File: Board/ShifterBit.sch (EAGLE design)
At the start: 13 parts, among them P1 PINHD-1X10, P2 PINHD-1X10

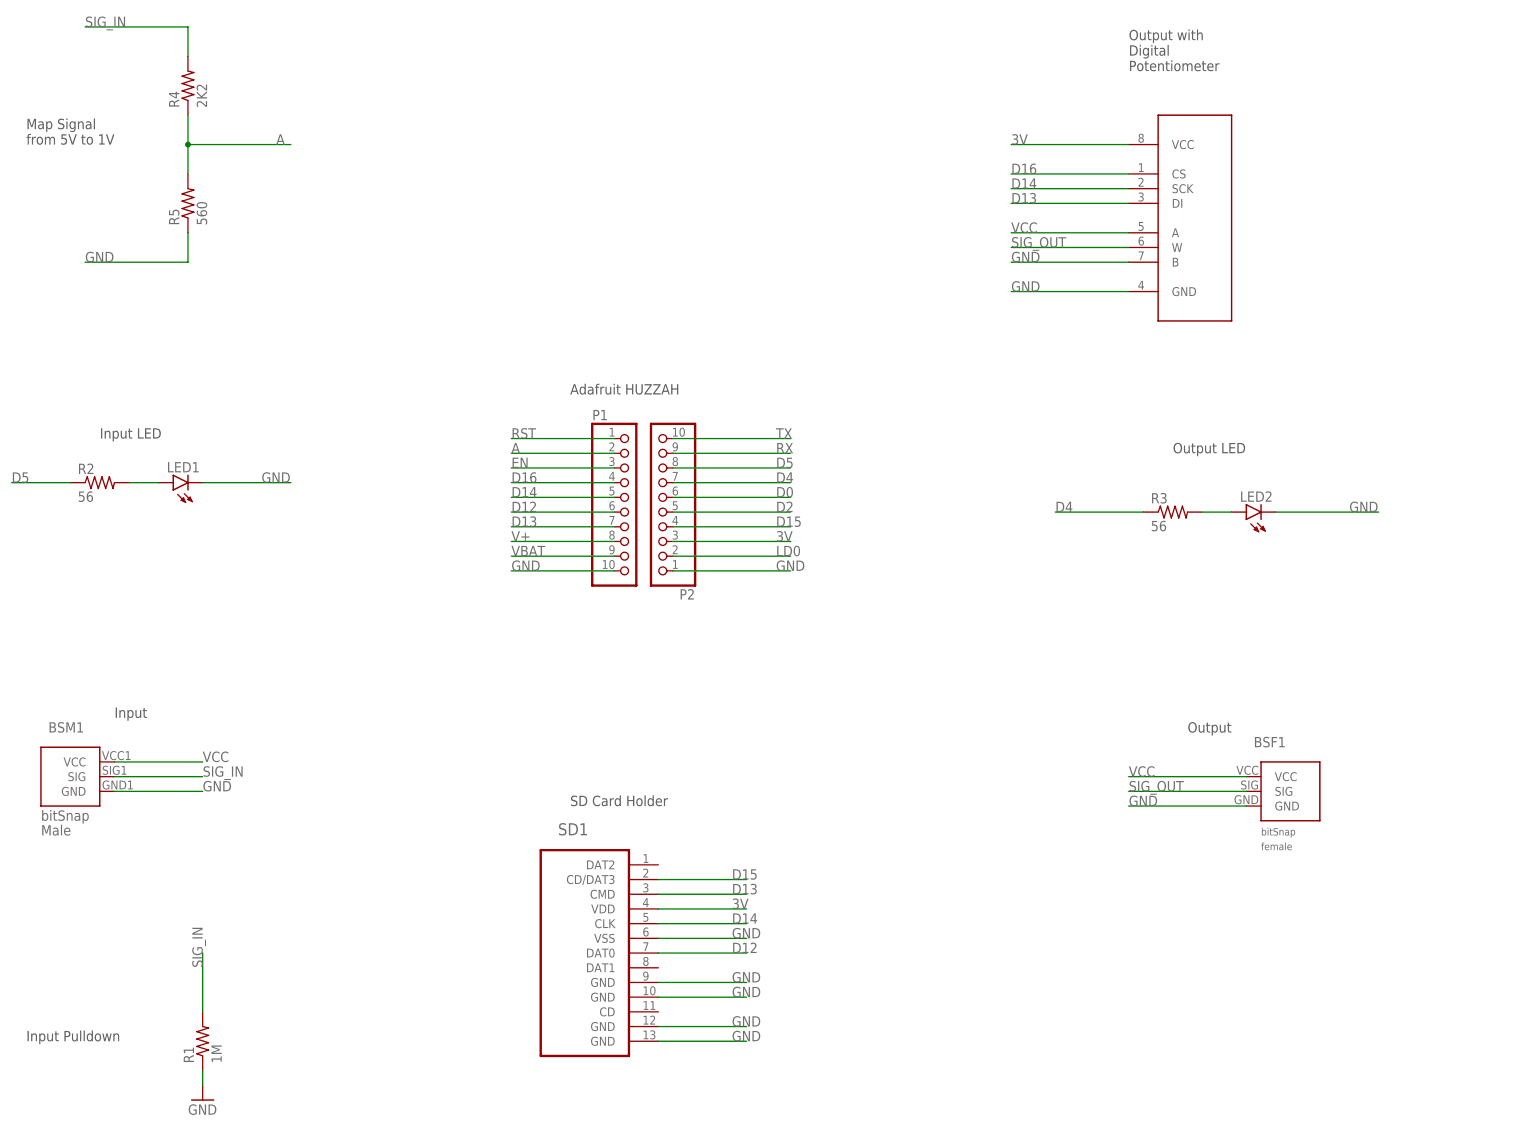
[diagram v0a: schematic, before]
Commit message: added some aesthetics
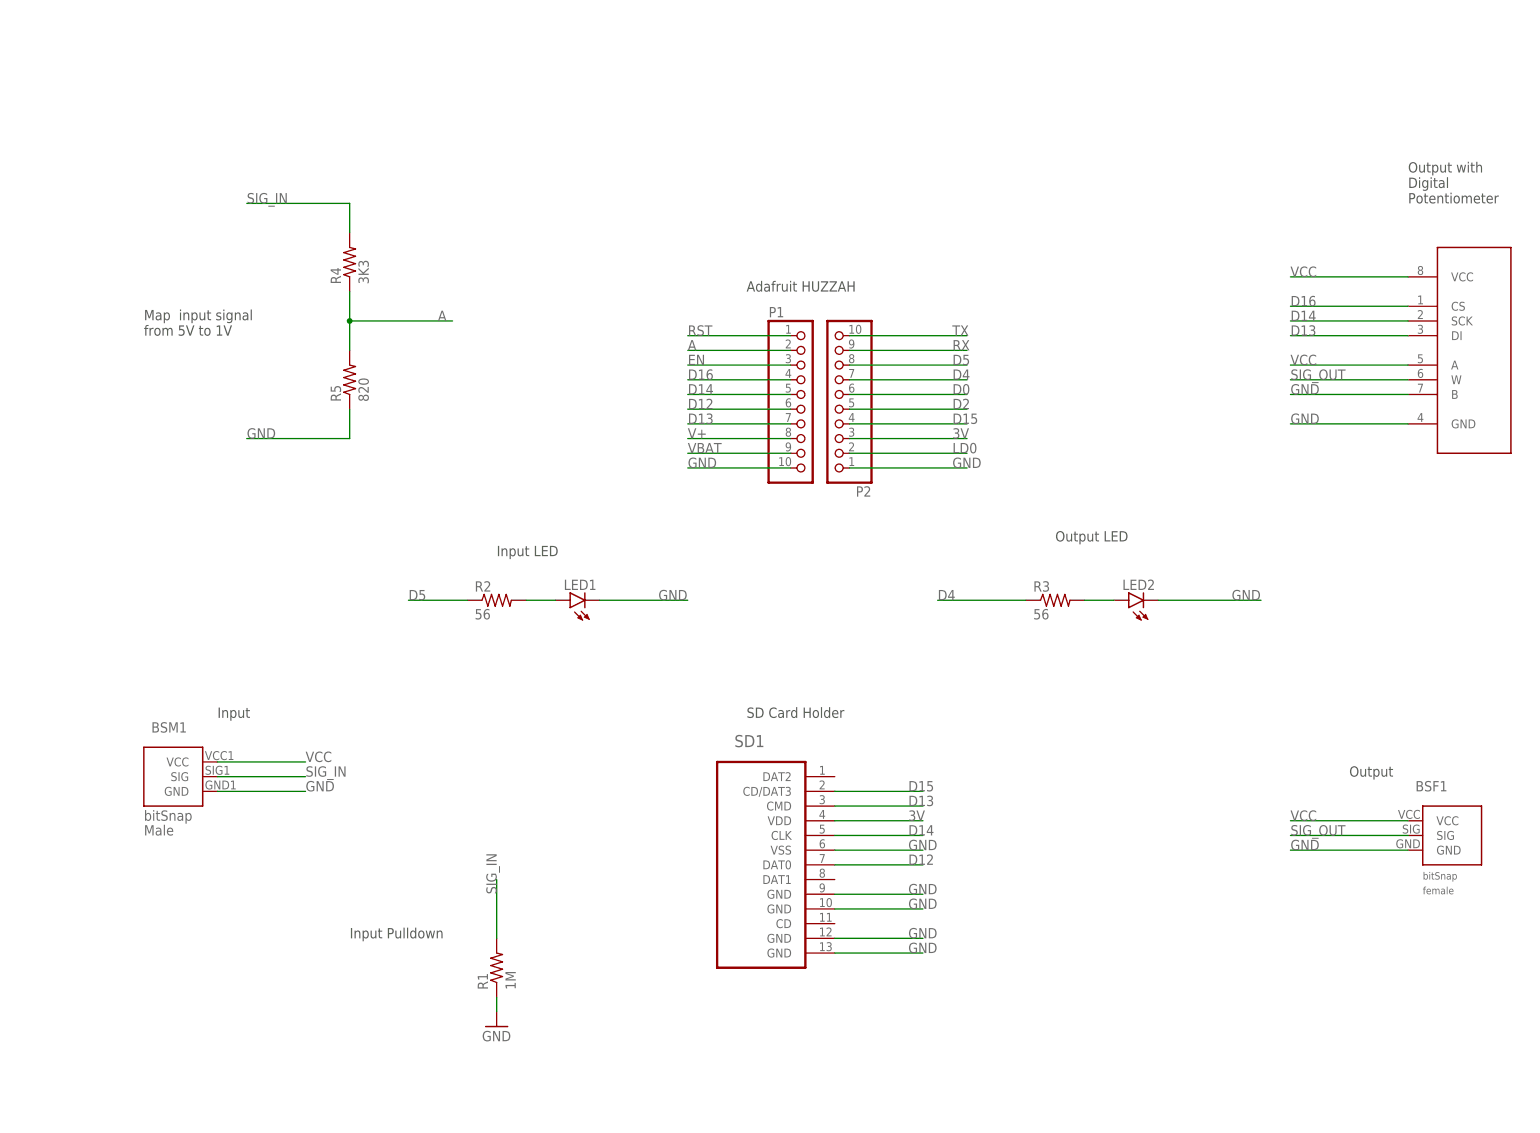
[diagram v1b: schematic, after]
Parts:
- R4: value 2K2 -> 3K3
- R5: value 560 -> 820
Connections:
- net 3V: no longer DPOT1.VCC
- net VCC: now also DPOT1.VCC
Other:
- note added: "Map input signal from 5V to 1V"
- note removed: "Map Signal from 5V to 1V"
- moved on the sheet: BSF1, BSM1, LED1, LED2, P1, P2, R1, R2, R3, R4, R5, SD1
